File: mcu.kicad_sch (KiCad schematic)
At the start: 31 parts, among them J2 DM3CS-SF, J4 SCREEN, U8 SiP32431DR3, U9 STM32F446RETx, Y1 X50328MSB2GI

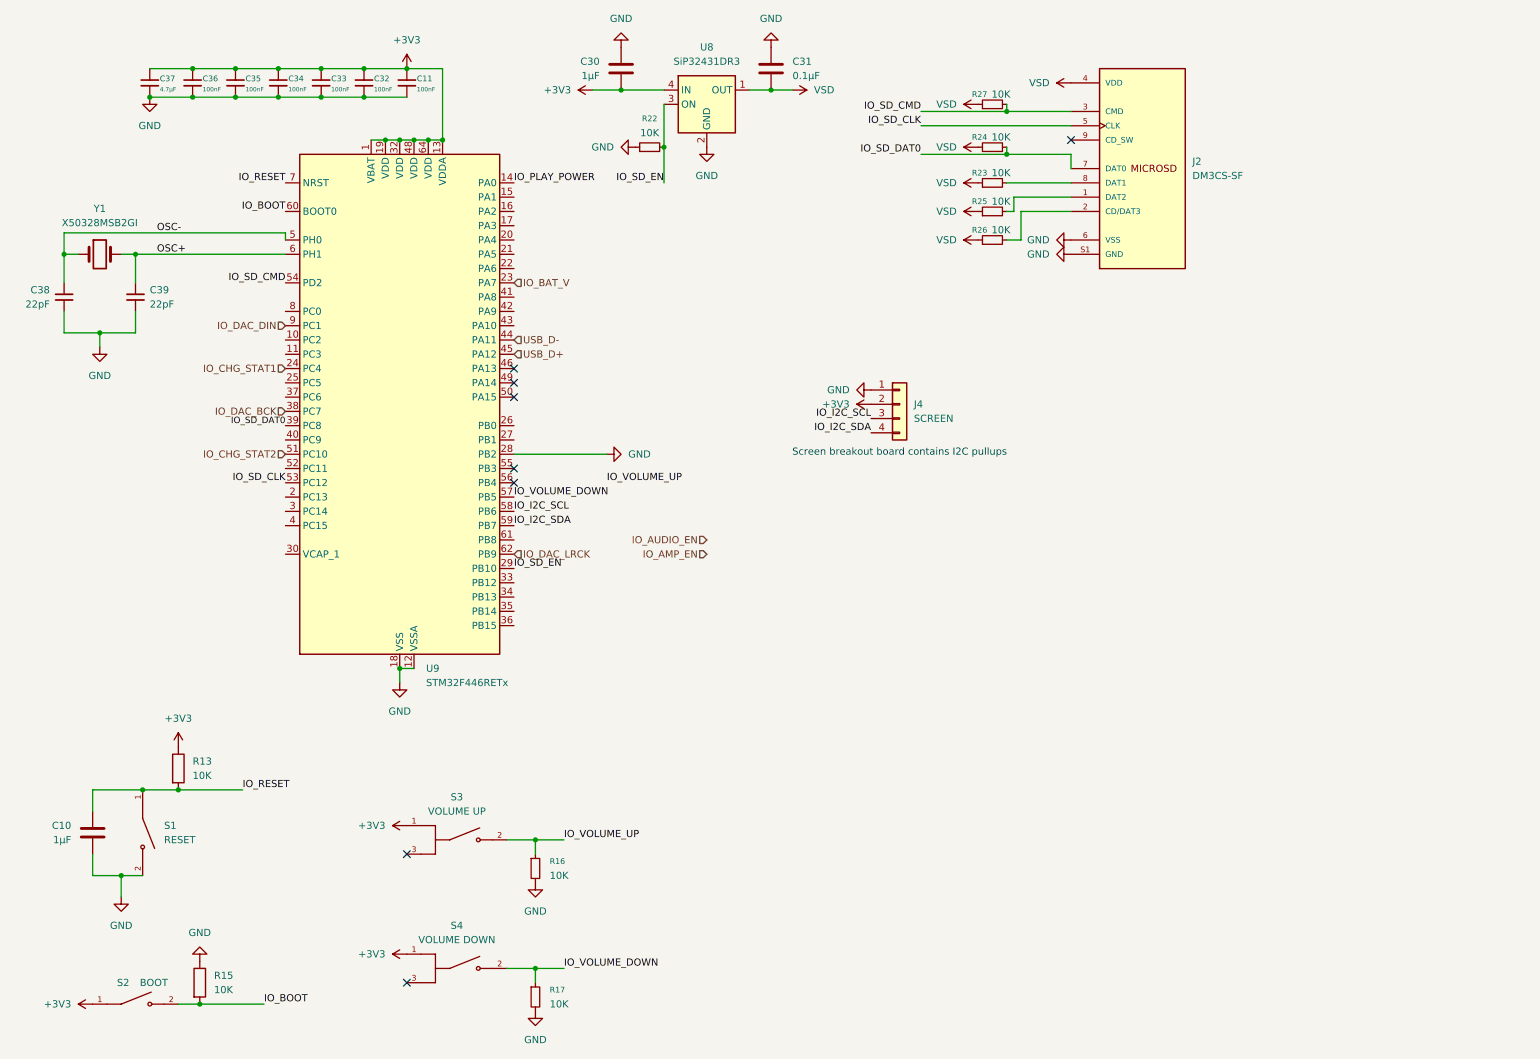
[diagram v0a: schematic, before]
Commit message: label sections
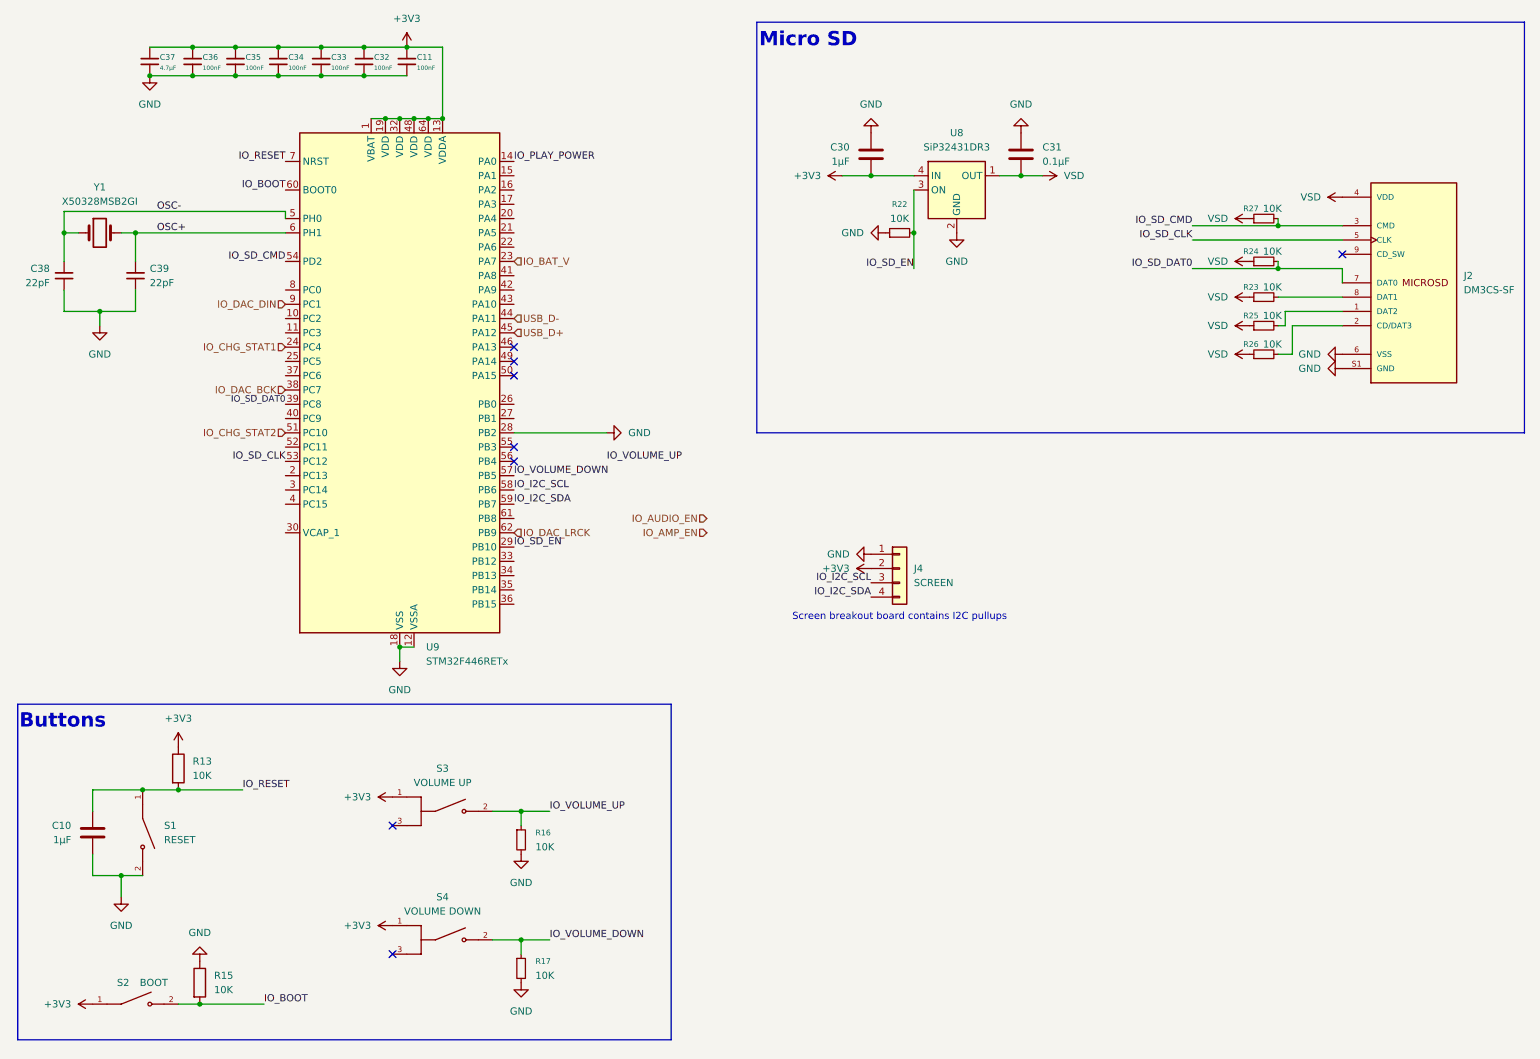
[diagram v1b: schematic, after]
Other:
- note added: "Buttons"
- note added: "Micro SD"
- moved on the sheet: C11, C30, C31, C32, C33, C34, C35, C36, C37, C38, C39, J2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
